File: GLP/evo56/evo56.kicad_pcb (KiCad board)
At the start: 2 copper layers, 138.8 x 106.7 mm, 67 parts

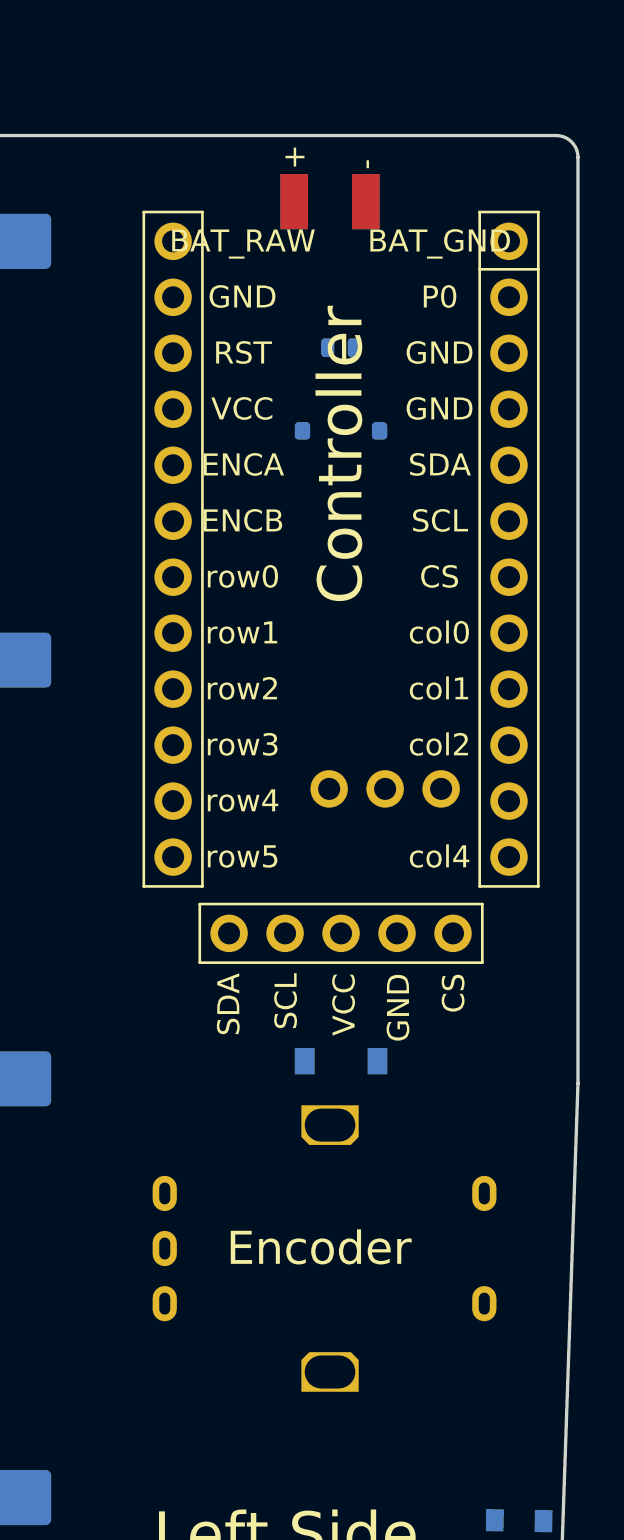
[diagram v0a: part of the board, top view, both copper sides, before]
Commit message: er i lied
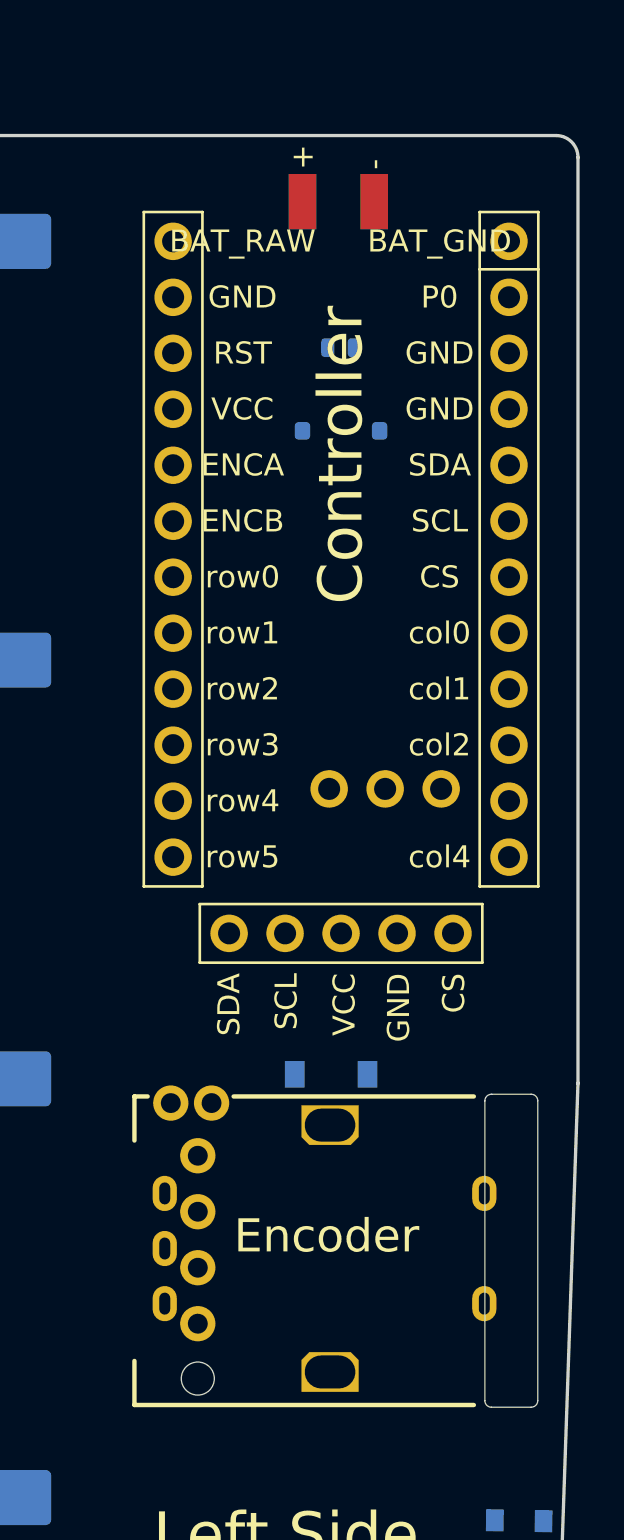
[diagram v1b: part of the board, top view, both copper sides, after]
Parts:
- added REF**: RollerEncoder_Panasonic_EVQWGD001, scrollwheel:RollerEncoder_Panasonic_EVQWGD001, F.Cu at (166.6, 114.1)
- moved D29 0.75 mm to (167.1, 106.6)
- moved PAD1 0.38 mm to (167.4, 67.0)
- moved G*** 0.20 mm to (167.0, 114.4)

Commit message: modularise more
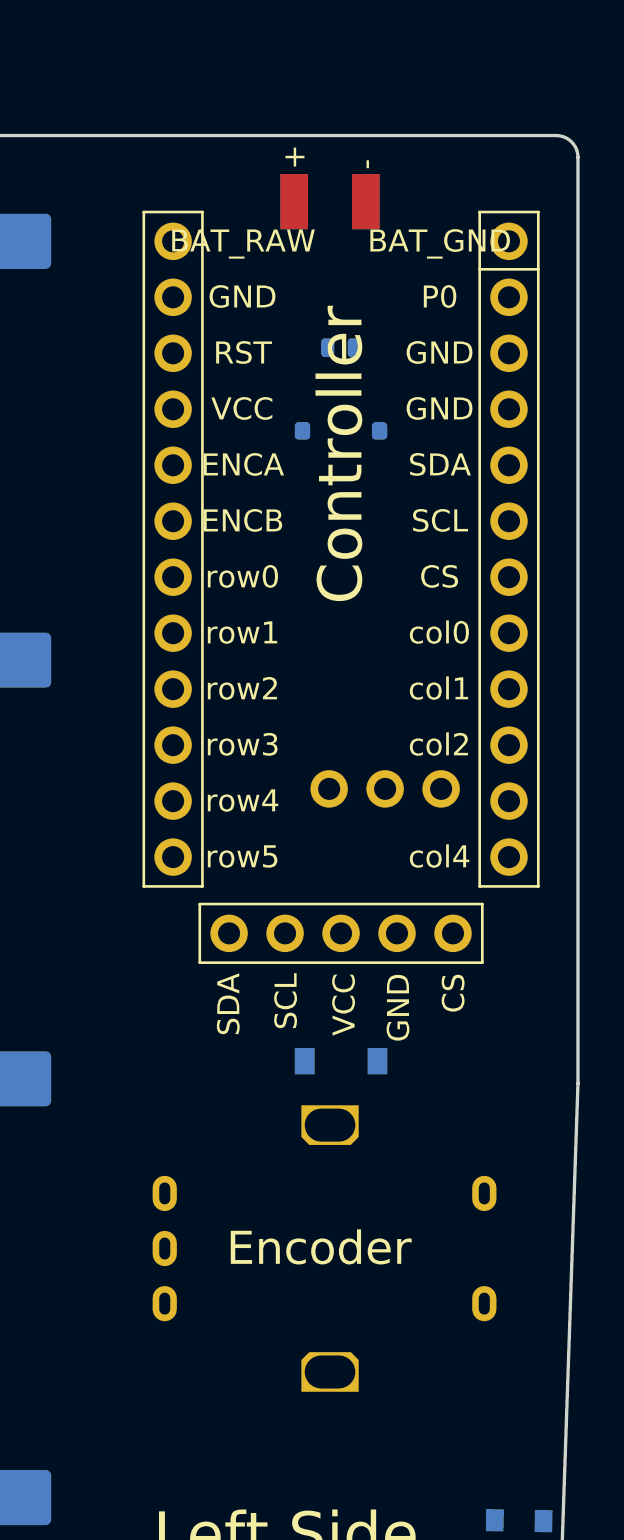
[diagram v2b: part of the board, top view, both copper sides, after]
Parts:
- removed REF**: RollerEncoder_Panasonic_EVQWGD001, scrollwheel:RollerEncoder_Panasonic_EVQWGD001
- moved D29 0.75 mm to (167.5, 106.0)
- moved PAD1 0.38 mm to (167.0, 67.0)
- moved G*** 0.20 mm to (167.0, 114.6)
